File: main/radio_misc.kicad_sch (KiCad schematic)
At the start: 23 parts, among them J601 Transponder, J602 Conn_01x03, J603 Conn_01x03, J604 Conn_01x03, J605 Conn_01x03, J606 Conn_01x03, J607 Conn_01x03, J608 USB_B_Micro, M601 Servo direction, Q601 IRLML0030, U601 FT230XQ

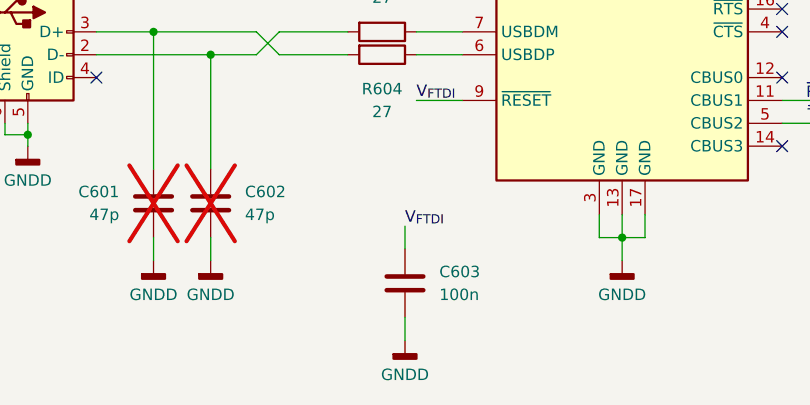
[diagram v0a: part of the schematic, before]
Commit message: Sent to fab
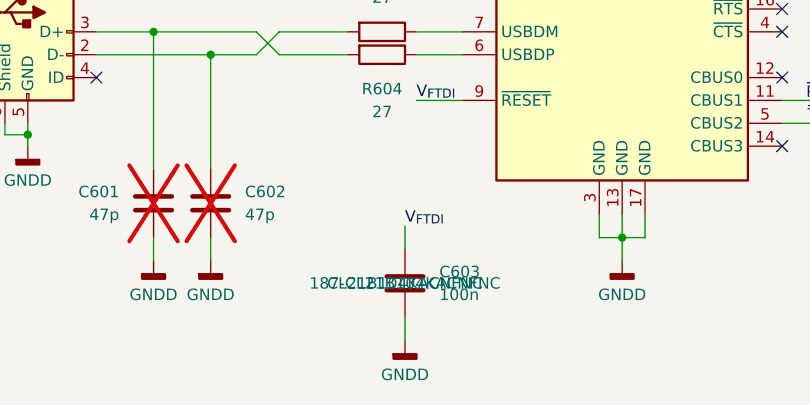
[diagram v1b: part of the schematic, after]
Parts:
- C603: MPN (none) -> CL21B104KACNFNC; Mouser SKU (none) -> 187-CL21B104KACNFNC
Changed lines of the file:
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@@
+			)
+		)
+		(property "Quantity" ""
+			(at 240.03 29.21 0)
+			(effects
+				(font
+					(size 1.27 1.27)
+				)
 			)
 		)
@@
 			)
 		)
+		(property "Quantity" ""
+			(at 132.08 60.96 0)
+			(effects
+				(font
+					(size 1.27 1.27)
+				)
+			)
+		)
 		(pin "3"
 		)
@@
 			)
 		)
+		(property "Quantity" ""
+			(at 105.41 60.96 0)
+			(effects
+				(font
+					(size 1.27 1.27)
+				)
+			)
+		)
 		(pin "3"
 		)
@@
 			)
 		)
+		(property "MPN" "CL21B104KACNFNC "
+			(at 113.03 158.75 0)
+			(effects
+				(font
+					(size 1.27 1.27)
+				)
+			)
+		)
+		(property "Mouser SKU" " 187-CL21B104KACNFNC "
+			(at 113.03 158.75 0)
+			(effects
+				(font
+					(size 1.27 1.27)
+				)
+			)
+		)
+		(property "Quantity" ""
+			(at 113.03 158.75 0)
+			(effects
+				(font
+					(size 1.27 1.27)
+				)
+			)
+		)
 		(pin "1"
 		)
@@
 			)
 		)
+		(property "Quantity" ""
+			(at 77.47 60.96 0)
+			(effects
+				(font
+					(size 1.27 1.27)
+				)
+			)
+		)
 		(pin "3"
 		)
@@
 			)
 		)
+		(property "Quantity" ""
+			(at 110.49 133.35 0)
+			(effects
+				(font
+					(size 1.27 1.27)
+				)
+			)
+		)
 		(pin "2"
 		)
@@
 			)
 		)
+		(property "Quantity" ""
+			(at 170.18 138.43 0)
+			(effects
+				(font
+					(size 1.27 1.27)
+				)
+			)
+		)
 		(pin "2"
 		)
@@
 			)
 		)
+		(property "Quantity" ""
+			(at 254 29.21 0)
+			(effects
+				(font
+					(size 1.27 1.27)
+				)
+			)
+		)
 		(pin "2"
 		)
@@
 			)
 		)
+		(property "Quantity" ""
+			(at 248.92 46.99 0)
+			(effects
+				(font
+					(size 1.27 1.27)
+				)
+			)
+		)
 		(pin "3"
 		)
@@
 			)
 		)
+		(property "Quantity" ""
+			(at 64.77 60.96 0)
+			(effects
+				(font
+					(size 1.27 1.27)
+				)
+			)
+		)
 		(pin "3"
 		)
@@
 			)
 		)
+		(property "Quantity" ""
+			(at 137.16 133.35 0)
+			(effects
+				(font
+					(size 1.27 1.27)
+				)
+			)
+		)
 		(pin "17"
 		)
@@
 			)
 		)
+		(property "Quantity" ""
+			(at 91.44 60.96 0)
+			(effects
+				(font
+					(size 1.27 1.27)
+				)
+			)
+		)
 		(pin "3"
 		)
@@
 			)
 		)
+		(property "Quantity" ""
+			(at 170.18 140.97 0)
+			(effects
+				(font
+					(size 1.27 1.27)
+				)
+			)
+		)
 		(pin "2"
 		)
@@
 			)
 		)
+		(property "Quantity" ""
+			(at 118.11 60.96 0)
+			(effects
+				(font
+					(size 1.27 1.27)
+				)
+			)
+		)
 		(pin "3"
 		)
@@
 			)
 		)
+		(property "Quantity" ""
+			(at 110.49 130.81 0)
+			(effects
+				(font
+					(size 1.27 1.27)
+				)
+			)
+		)
 		(pin "2"
 		)
@@
 				)
 				(hide yes)
+			)
+		)
+		(property "Quantity" ""
+			(at 191.77 127 0)
+			(effects
+				(font
+					(size 1.27 1.27)
+				)
 			)
 		)
@@
 			)
 		)
+		(property "Quantity" ""
+			(at 91.44 22.86 0)
+			(effects
+				(font
+					(size 1.27 1.27)
+				)
+			)
+		)
 		(pin "1"
 		)
@@
 			)
 		)
+		(property "Quantity" ""
+			(at 49.53 60.96 0)
+			(effects
+				(font
+					(size 1.27 1.27)
+				)
+			)
+		)
 		(pin "3"
 		)
@@
 			)
 		)
+		(property "Quantity" ""
+			(at 85.09 149.86 0)
+			(effects
+				(font
+					(size 1.27 1.27)
+				)
+			)
+		)
 		(pin "1"
 		)
@@
 			)
 		)
+		(property "Quantity" ""
+			(at 71.12 130.81 0)
+			(effects
+				(font
+					(size 1.27 1.27)
+				)
+			)
+		)
 		(pin "5"
 		)
@@
 			)
 		)
+		(property "Quantity" ""
+			(at 91.44 149.86 0)
+			(effects
+				(font
+					(size 1.27 1.27)
+				)
+			)
+		)
 		(pin "1"
 		)
@@
 			)
 		)
+		(property "Quantity" ""
+			(at 240.03 52.07 0)
+			(effects
+				(font
+					(size 1.27 1.27)
+				)
+			)
+		)
 		(pin "2"
 		)
@@
 			)
 		)
+		(property "Quantity" ""
+			(at 207.01 127 0)
+			(effects
+				(font
+					(size 1.27 1.27)
+				)
+			)
+		)
